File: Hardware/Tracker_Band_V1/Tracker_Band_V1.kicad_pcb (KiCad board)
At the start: 4 copper layers, 18.5 x 30 mm, 52 parts, among them J1 USB_C_USB20, Q1 SSM6L56FE, SW1 EVP-AVAA1A, SW2 EVP-AVAA1A, U1 ESP32-C3-MINI-1-N4, U2 BNO085, U3 RT8010, U4 MCP73832-2-AC, U5 LM66200, U6 IN-PI15TAT5R5G5B, U7 IN-PI15TAT5R5G5B, U8 IN-PI15TAT5R5G5B, U9 IN-PI15TAT5R5G5B, X1 32.768kHz

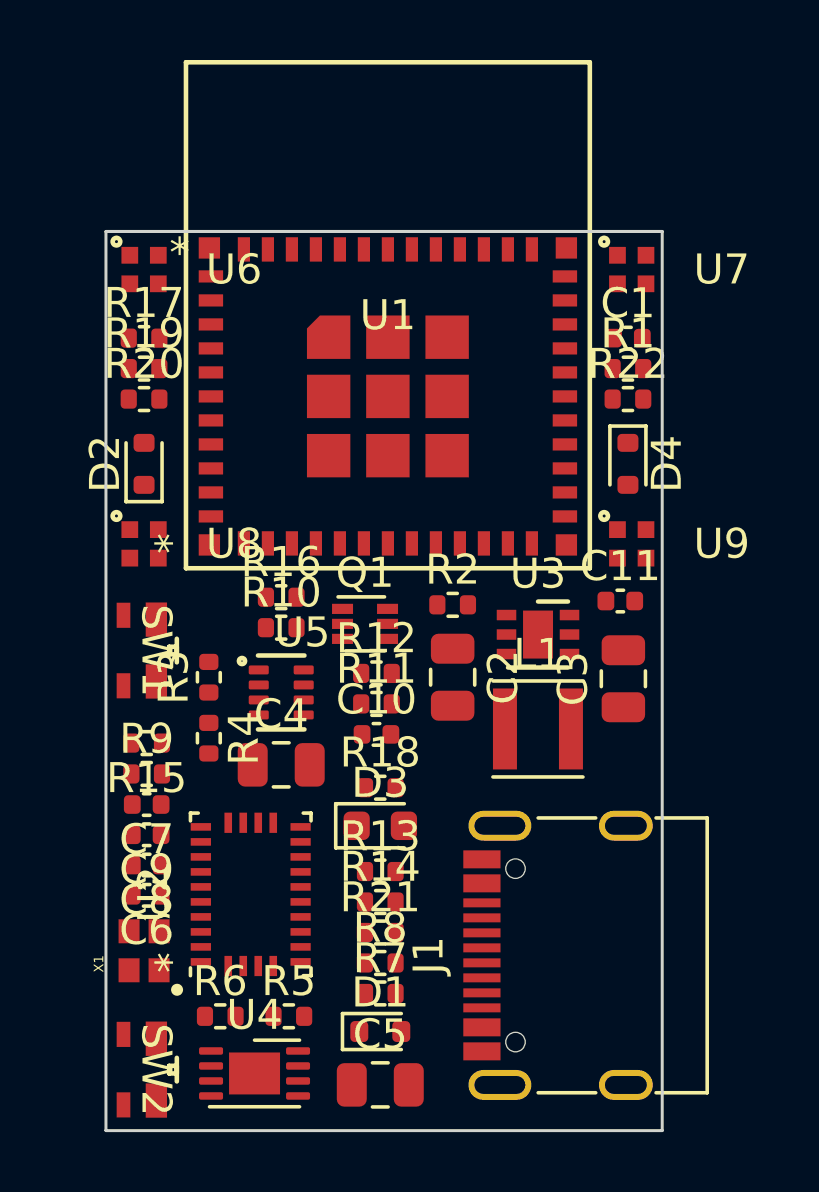
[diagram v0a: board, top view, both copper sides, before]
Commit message: Component positioning & PCB sizing
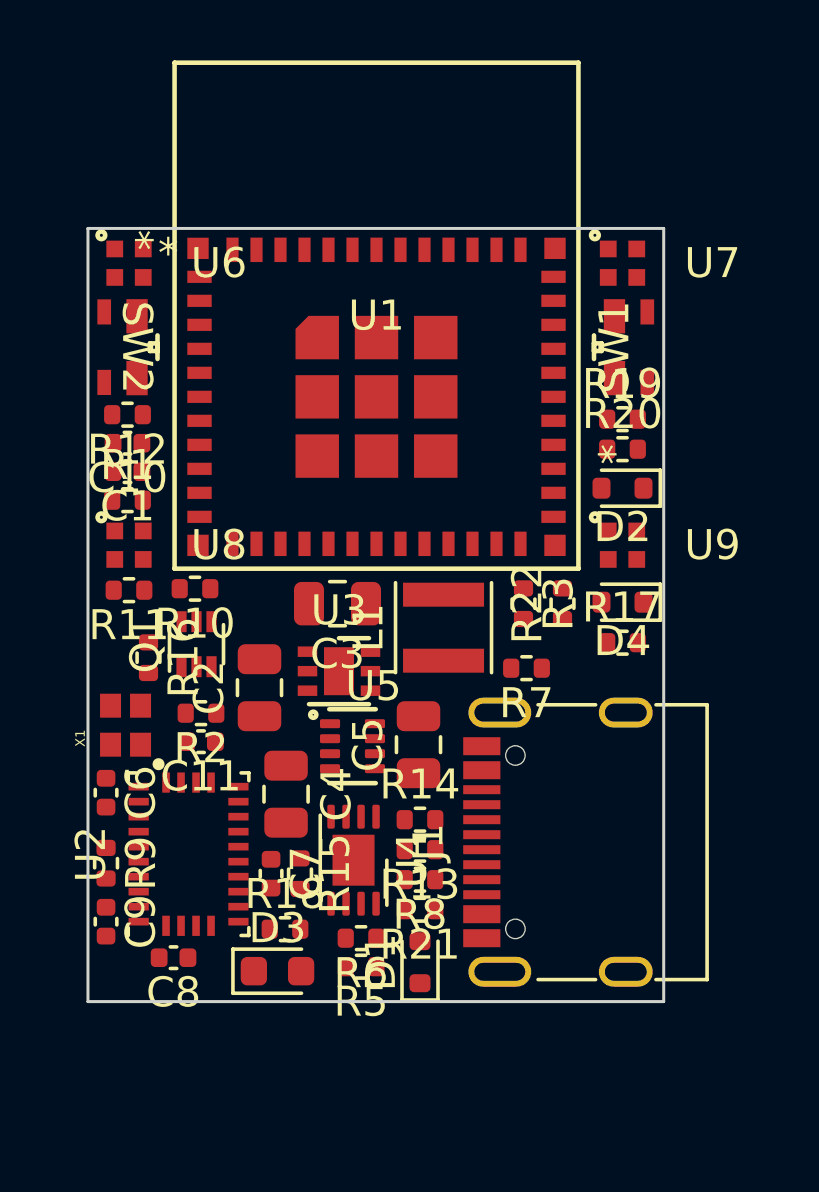
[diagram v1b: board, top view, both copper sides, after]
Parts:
- removed R4: 10k, Resistor_SMD:R_0402_1005Metric
- R22: value 100k -> 1k
- moved SW2 24.1 mm to (122.8, 79.5)
- moved SW1 19.9 mm to (140.6, 79.5), turned to 90 degrees
- moved R17 18.9 mm to (139.9, 89.4)
- moved C1 17.3 mm to (123.4, 83.7), turned to 180 degrees
- moved R1 17.2 mm to (123.4, 84.7)
- moved R19 16.0 mm to (139.9, 82.0)
- moved R20 16.0 mm to (139.9, 83.0)
- moved D2 16.0 mm to (139.9, 84.2), turned to 180 degrees
- moved C11 14.7 mm to (125.8, 92.7), turned to 180 degrees
- moved C10 12.8 mm to (123.4, 82.8), turned to 180 degrees
- moved R12 12.0 mm to (123.4, 81.8), turned to 180 degrees
- moved R7 11.9 mm to (136.7, 90.2), turned to 180 degrees
- moved C5 11.4 mm to (133.1, 92.8), turned to 90 degrees
- moved R3 10.8 mm to (136.6, 88.1), turned to -90 degrees
- moved C3 9.85 mm to (130.4, 88.1), turned to 180 degrees
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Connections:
- net Net-(U6-DOUT) renamed /RGB_LED1
- net Net-(U7-DOUT) renamed /RGB_LED2
- net Net-(U8-DOUT) renamed /RGB_LED3
- R17 pad 2: Net-(R17-Pad2) -> Net-(SW1-A)
- SW1 pad 1: Net-(R17-Pad2) -> Net-(D2-A)
- SW1 pad 2: unconnected-(SW1-Pad2) -> Net-(D2-A)
- SW1 pad 4: Net-(D2-A) -> Net-(SW1-A)
- U1 pad 6: unconnected-(U1-GPIO3,_ADC1_CH3-Pad6) -> /VBAT_ADC
- U3 pad 7: (no net) -> GND
- U4 pad 9: (no net) -> GND
- U5 pad 4: Net-(U5-~{ON}) -> GND
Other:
- board size 18.5 x 30 mm -> 19.2 x 25.8 mm
